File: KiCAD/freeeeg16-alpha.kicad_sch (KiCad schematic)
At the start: 23 parts, among them J1 Conn_02x03_Odd_Even, J28 Conn_02x03_Odd_Even, J29 Conn_02x03_Odd_Even, J30 Conn_02x03_Odd_Even, J31 Conn_02x03_Odd_Even, J32 Conn_02x03_Odd_Even, J33 Conn_02x03_Odd_Even, J5 Conn_01x07, J6 Conn_01x06, SW1 SW_Push, SW2 SW_Push, SW3 SW_Push, SW4 SW_Push

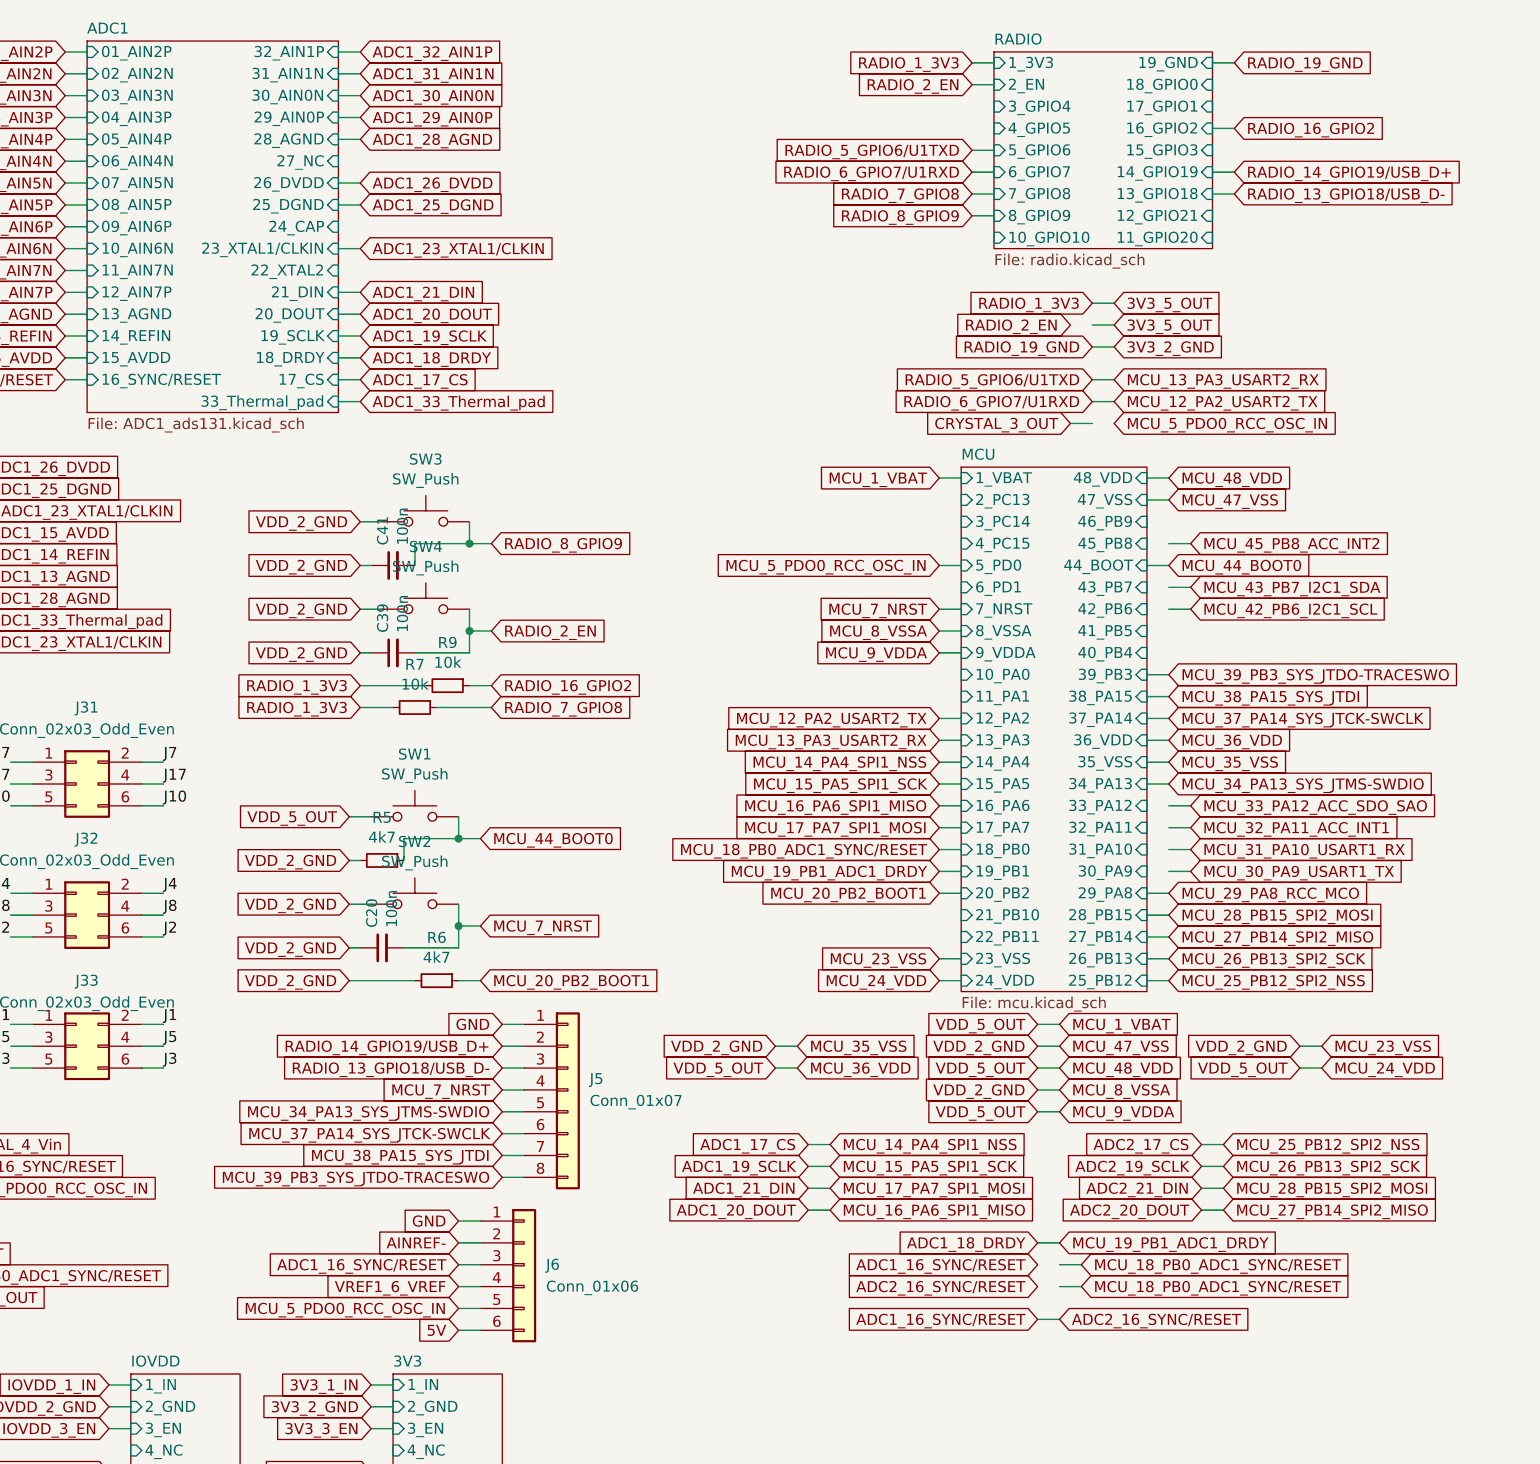
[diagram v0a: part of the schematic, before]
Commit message: Add files via upload
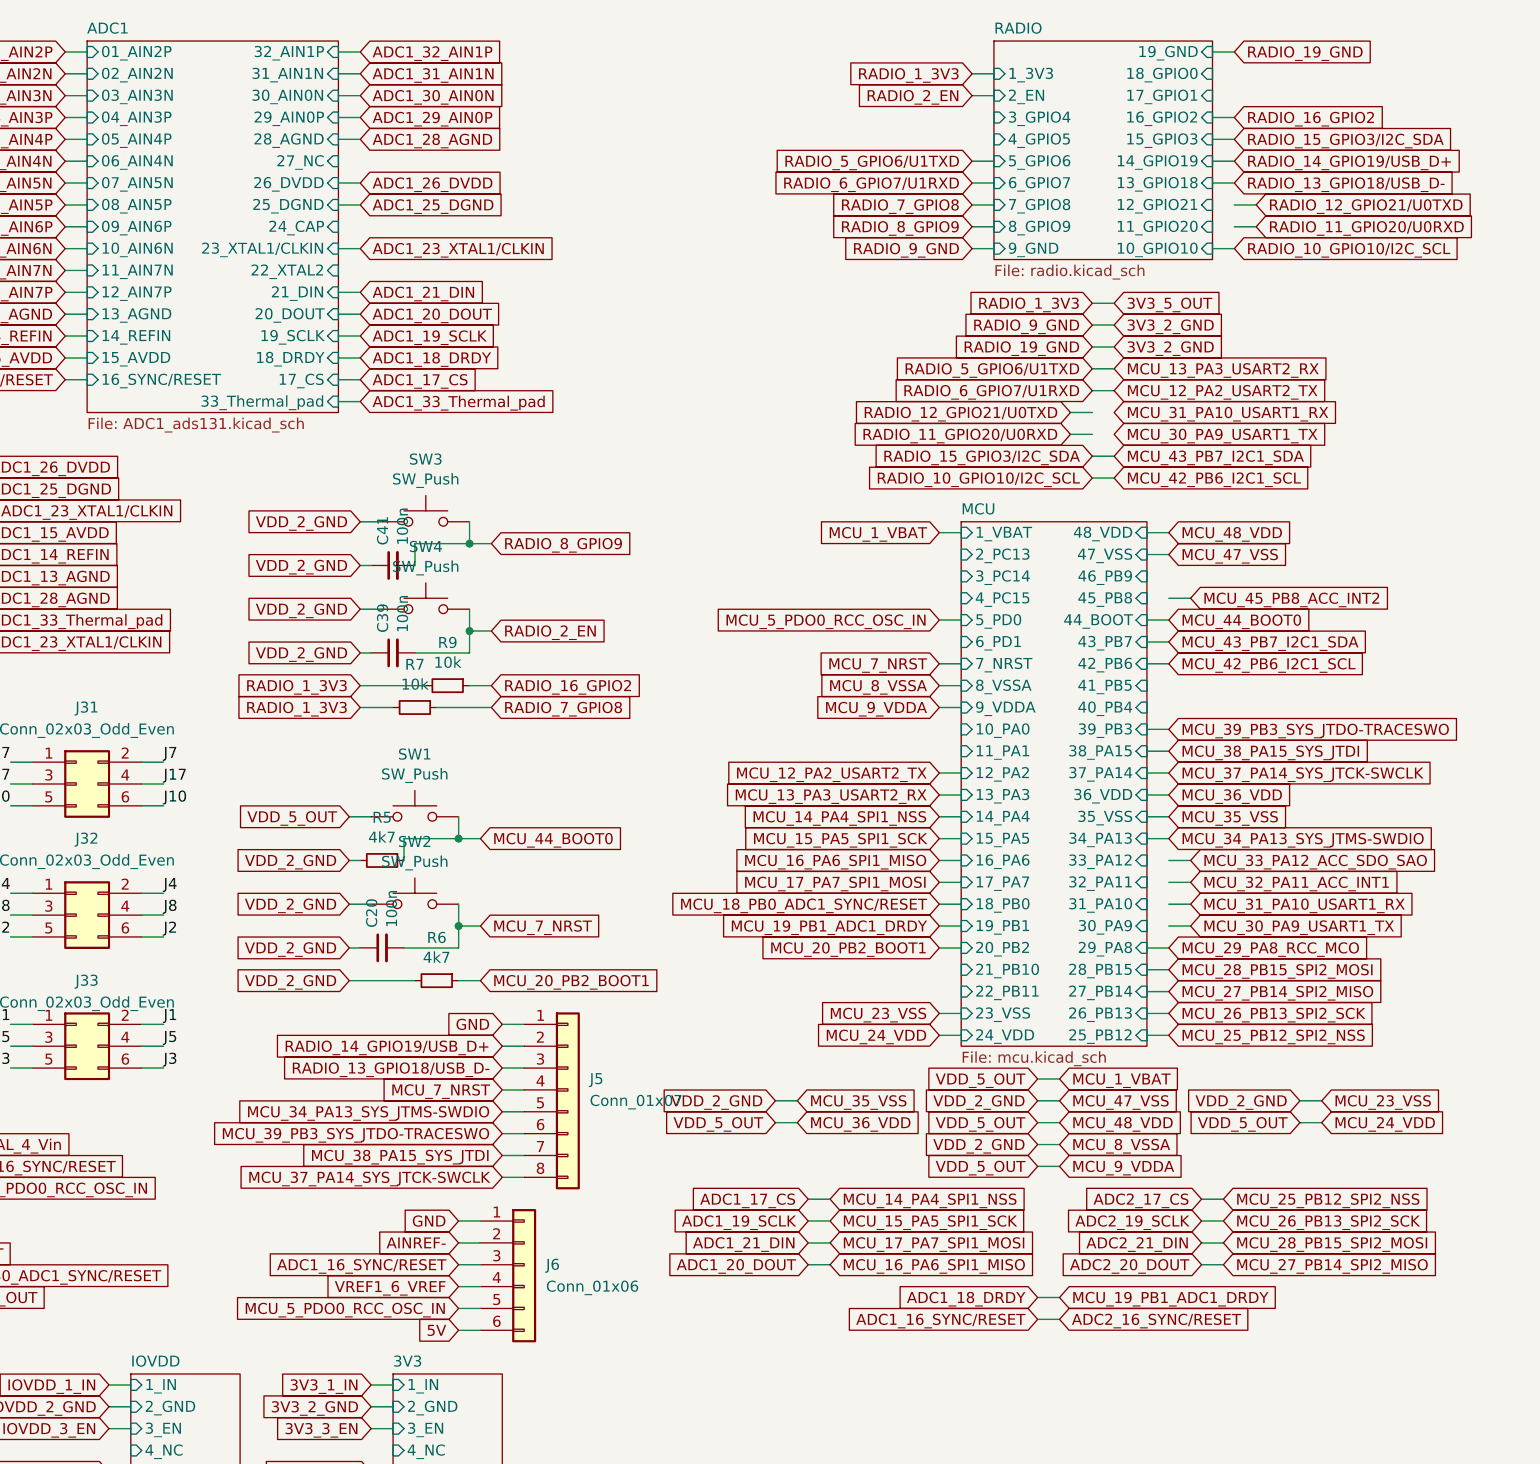
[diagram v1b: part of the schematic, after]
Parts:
- J5: footprint Connector_Molex:Molex_PicoBlade_53398-0771_1x07-1MP_P1.25mm_Vertical -> freeeeg16:Molex_PicoBlade_53398-0871_1x08-1MP_P1.25mm_Vertical_cut
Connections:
- net MCU_37_PA14_SYS_JTCK-SWCLK: now also J5.8 (Pin_8); no longer J5.6 (Pin_6)
- net MCU_39_PB3_SYS_JTDO-TRACESWO: now also J5.6 (Pin_6); no longer J5.8 (Pin_8)
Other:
- sheet RADIO ports: added 9_GND; removed none

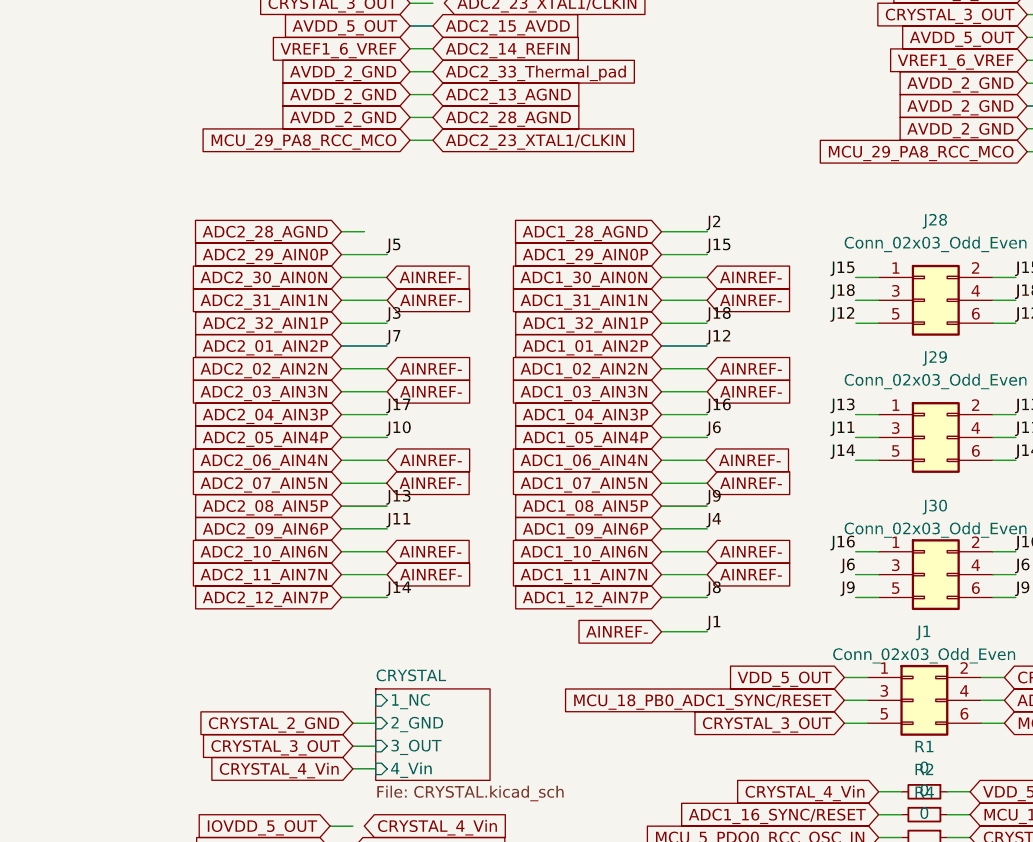
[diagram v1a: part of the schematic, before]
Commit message: Add files via upload
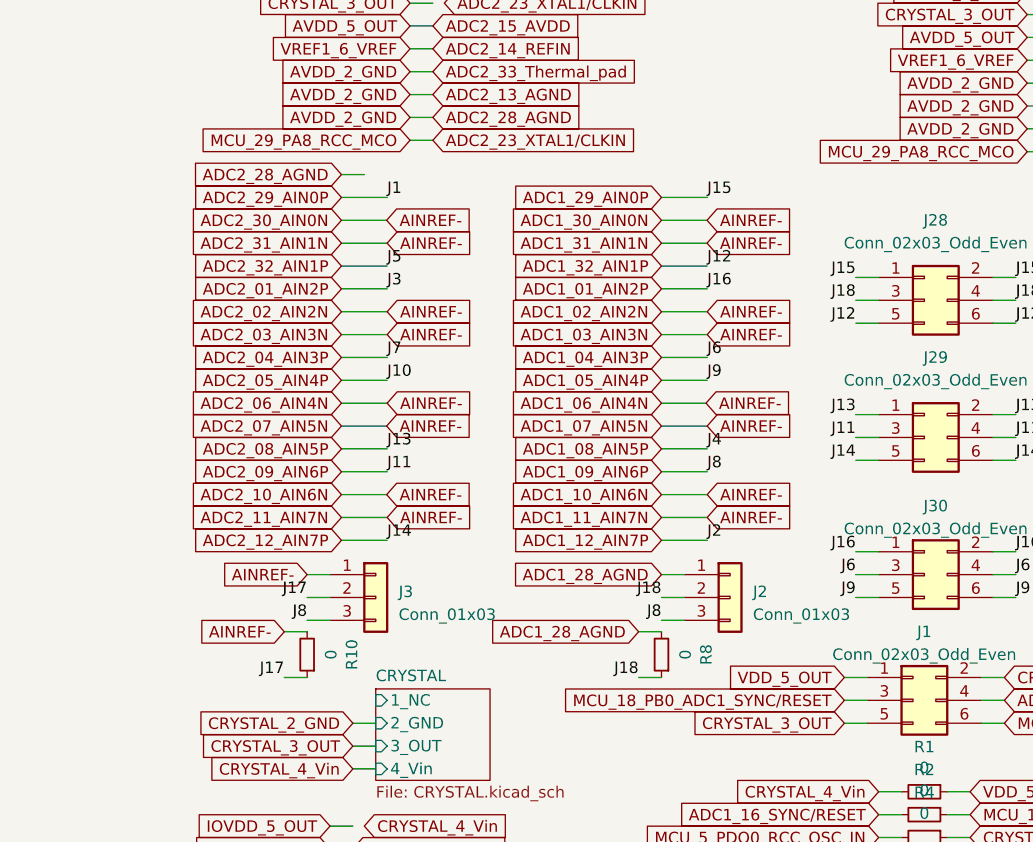
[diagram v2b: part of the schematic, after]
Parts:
- added J2, J3: Conn_01x03, Connector_PinHeader_1.27mm:PinHeader_1x03_P1.27mm_Vertical, symbol Connector_Generic:Conn_01x03
- added R10, R8: 0, Resistor_SMD:R_0402_1005Metric, symbol FreeEEG32-ads131-rescue:R_Small-Device
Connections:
- net 3V3_2_GND: now also J2.1 (Pin_1), R8.2; no longer J32.5 (Pin_5), J32.6 (Pin_6)
- net ADC1_01_AIN2P: now also J30.1 (Pin_1), J30.2 (Pin_2); no longer J28.5 (Pin_5), J28.6 (Pin_6)
- net ADC1_02_AIN2N: now also J3.1 (Pin_1), R10.2; no longer J33.1 (Pin_1), J33.2 (Pin_2)
- net ADC1_04_AIN3P: now also J30.3 (Pin_3), J30.4 (Pin_4); no longer J30.1 (Pin_1), J30.2 (Pin_2)
- net ADC1_05_AIN4P: now also J30.5 (Pin_5), J30.6 (Pin_6); no longer J30.3 (Pin_3), J30.4 (Pin_4)
- net ADC1_08_AIN5P: now also J32.1 (Pin_1), J32.2 (Pin_2); no longer J30.5 (Pin_5), J30.6 (Pin_6)
- net ADC1_09_AIN6P: now also J32.3 (Pin_3), J32.4 (Pin_4), J2.3 (Pin_3), J3.3 (Pin_3); no longer J32.1 (Pin_1), J32.2 (Pin_2)
- net ADC1_12_AIN7P: now also J32.5 (Pin_5), J32.6 (Pin_6); no longer J32.3 (Pin_3), J32.4 (Pin_4)
- net ADC1_32_AIN1P: now also J28.5 (Pin_5), J28.6 (Pin_6); no longer J28.3 (Pin_3), J28.4 (Pin_4)
- net ADC2_01_AIN2P: now also J33.5 (Pin_5), J33.6 (Pin_6); no longer J31.1 (Pin_1), J31.2 (Pin_2)
- net ADC2_04_AIN3P: now also J31.1 (Pin_1), J31.2 (Pin_2); no longer J31.3 (Pin_3), J31.4 (Pin_4)
- net ADC2_29_AIN0P: now also J33.1 (Pin_1), J33.2 (Pin_2); no longer J33.3 (Pin_3), J33.4 (Pin_4)
- net ADC2_32_AIN1P: now also J33.3 (Pin_3), J33.4 (Pin_4); no longer J33.5 (Pin_5), J33.6 (Pin_6)
- new net J17: J3.2 (Pin_2), J31.3 (Pin_3), J31.4 (Pin_4), R10.1
- new net J18: J2.2 (Pin_2), J28.3 (Pin_3), J28.4 (Pin_4), R8.1
